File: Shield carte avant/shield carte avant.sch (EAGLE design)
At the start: 29 parts, among them IC1 MCP2562-E_P, IC2 MCP2515-I_P, J1 22-05-7078-07, J2 22-05-7028-02, J3 22-05-7038-03, J5 22-05-7028-02, M1 ARDUINO_R3_ICSP

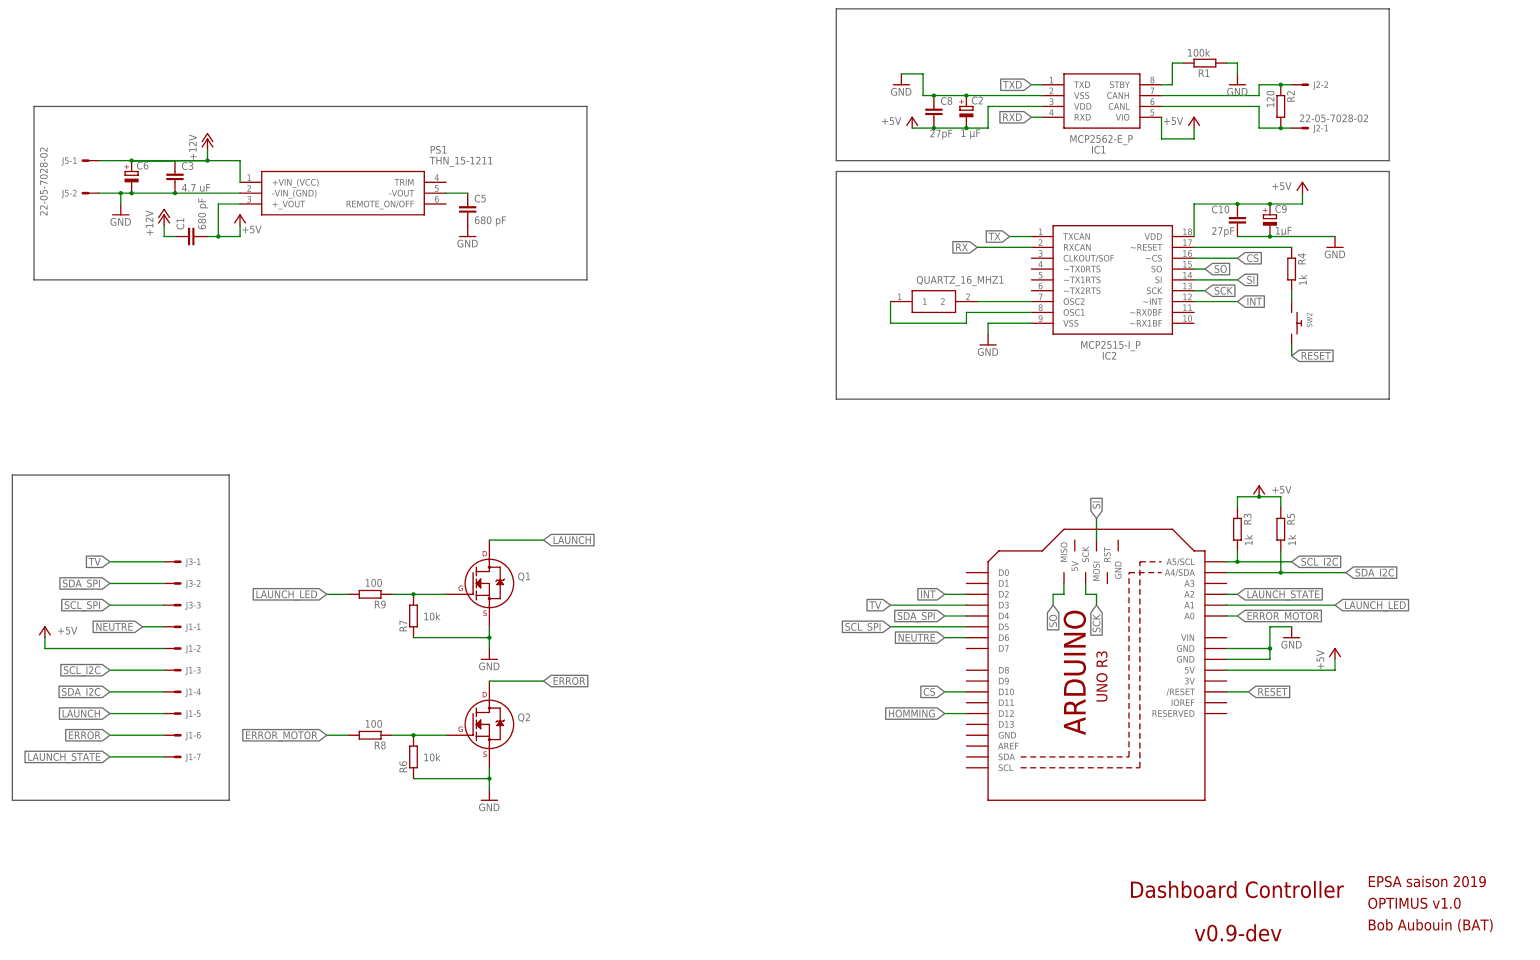
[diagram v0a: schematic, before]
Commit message: Fin du routage et vérification sérigraphie
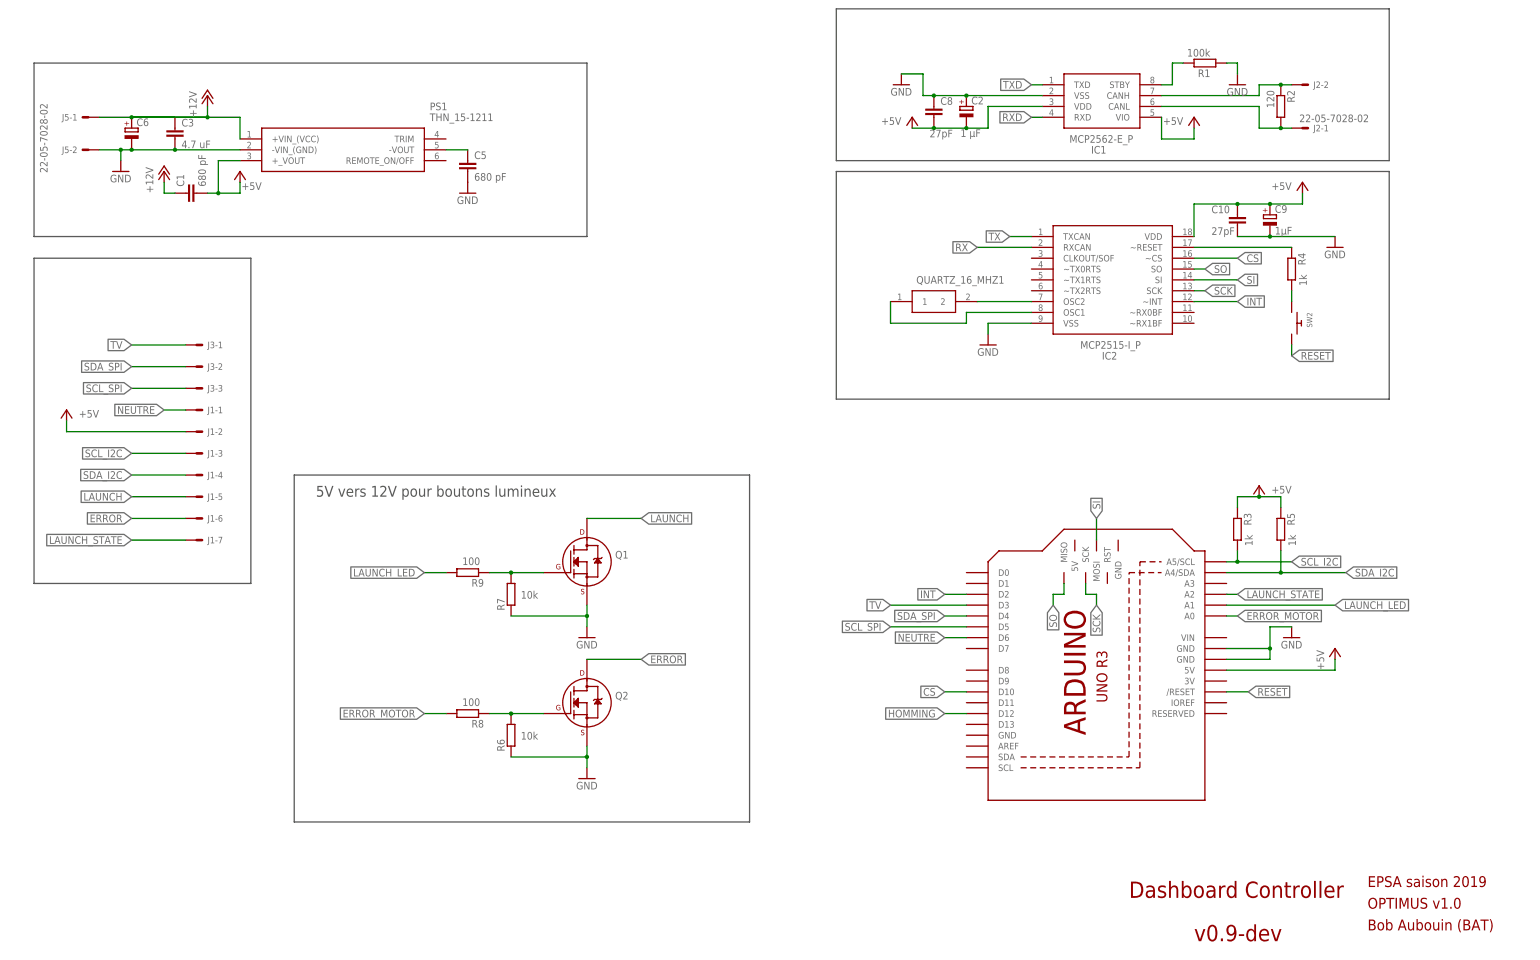
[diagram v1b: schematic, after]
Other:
- note added: "5V vers 12V pour boutons lumineux"
- moved on the sheet: C1, C3, C5, C6, J1-1, J1-2, J1-3, J1-4, J1-5, J1-6, J1-7, J3-1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
